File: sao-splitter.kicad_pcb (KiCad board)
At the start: 2 copper layers, 66 x 47.3 mm, 7 parts

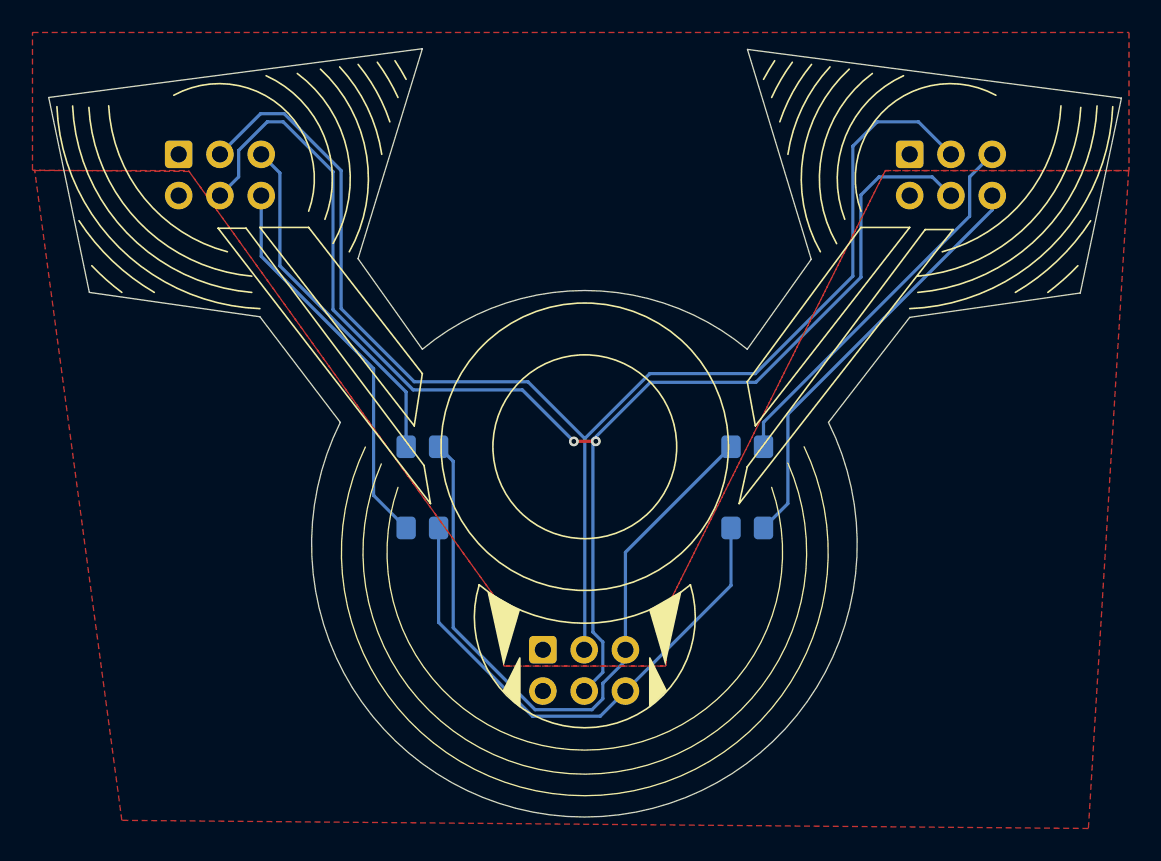
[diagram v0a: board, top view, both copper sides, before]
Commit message: Make smaller
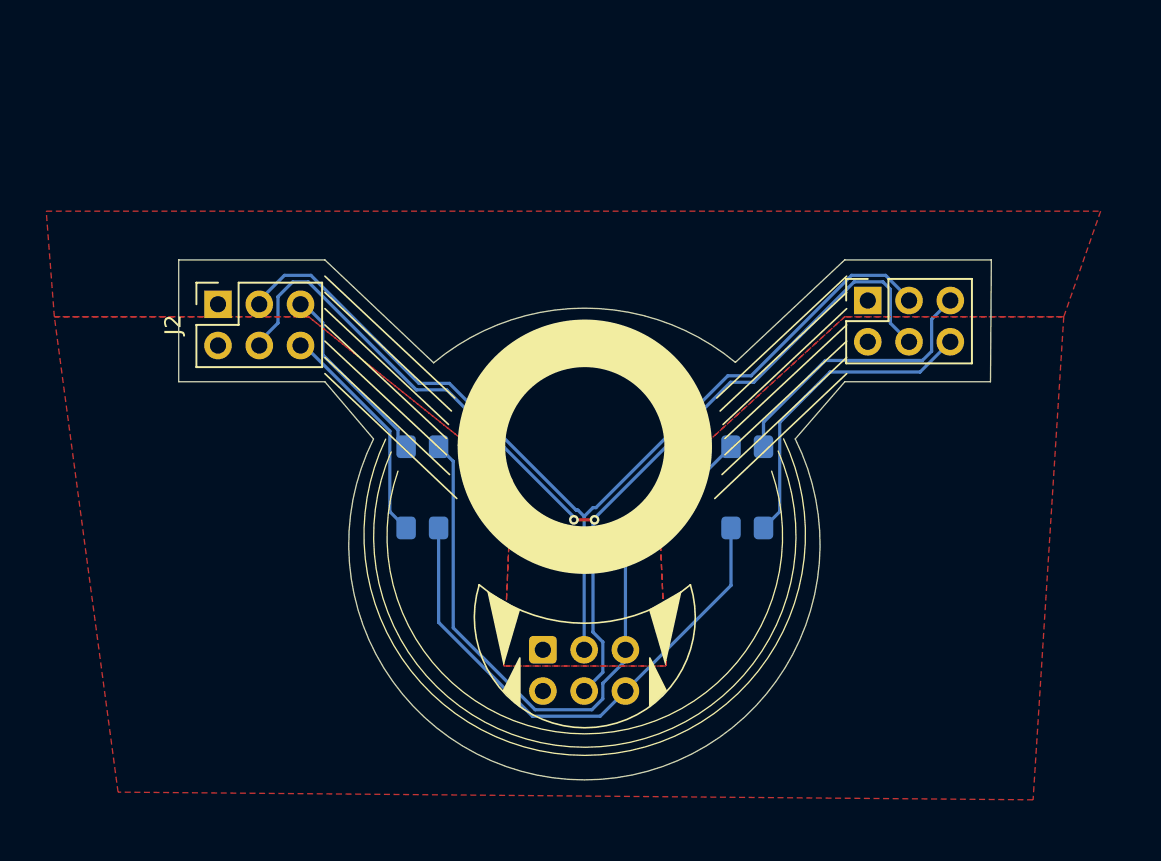
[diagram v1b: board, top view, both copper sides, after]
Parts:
- J2, J3: footprint Library:IDC-Header_2x03_P2.54mm_Vertical_SilkscreenHidden -> Connector_PinSocket_2.54mm:PinSocket_2x03_P2.54mm_Vertical; moved to F.Cu
- R1, R2, R3, R4: value 330 -> 330Ω
- moved J2 9.54 mm to (152.4, 109.2), turned to 90 degrees
- moved J3 9.36 mm to (192.4, 109.0), turned to 90 degrees
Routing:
- net /SDA: track 85.9 -> 61.9 mm
- net /SCL: track 87.7 -> 68.8 mm
- net Net-(J2-Pin_6): track 24.2 -> 14.2 mm
- net Net-(J2-Pin_5): track 21.7 -> 11.7 mm
- net Net-(J3-Pin_6): track 26.3 -> 19.5 mm
- net Net-(J3-Pin_5): track 23.8 -> 17.3 mm
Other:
- board size 66 x 47.3 mm -> 50 x 32 mm
- board text added: "GPIO1"
- board text added: "GPIO2"
- board text added: "https://github.com/bwasserm/ sao-spectator-splitter"
- board text removed: "https://github.com/bwasserm/sao-spectator-splitter"
